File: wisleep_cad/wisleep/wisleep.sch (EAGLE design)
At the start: 23 parts, among them IC1 STM32F10XCXT6, U1 MAX1555, X1 8MHz

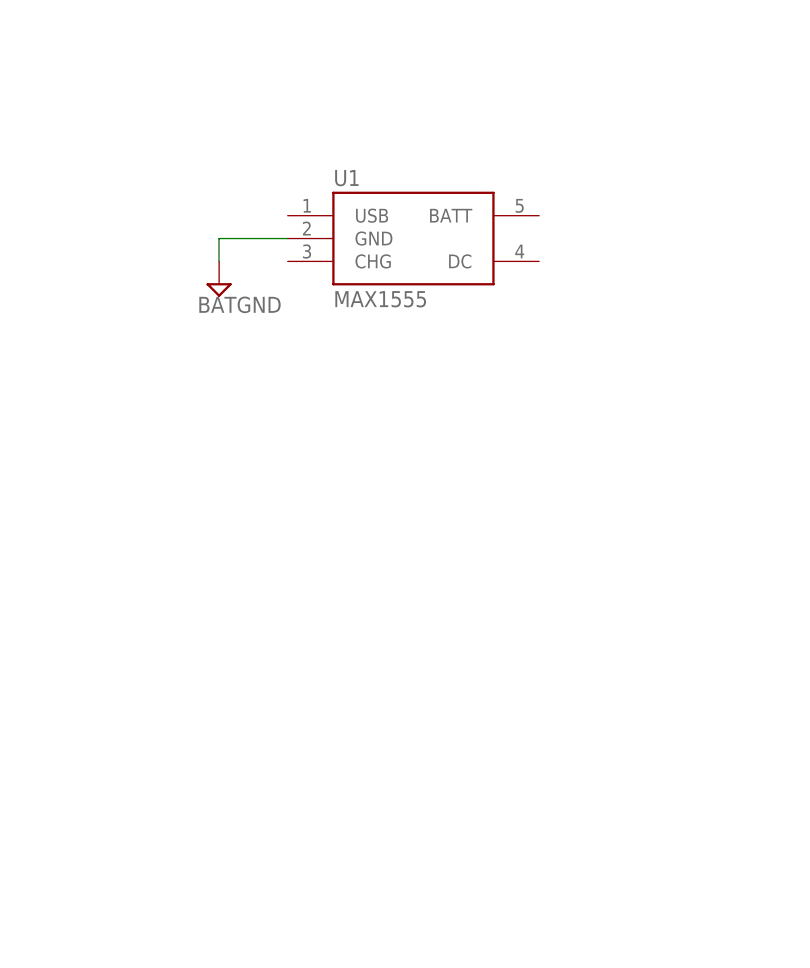
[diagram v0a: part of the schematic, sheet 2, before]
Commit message: some more cad
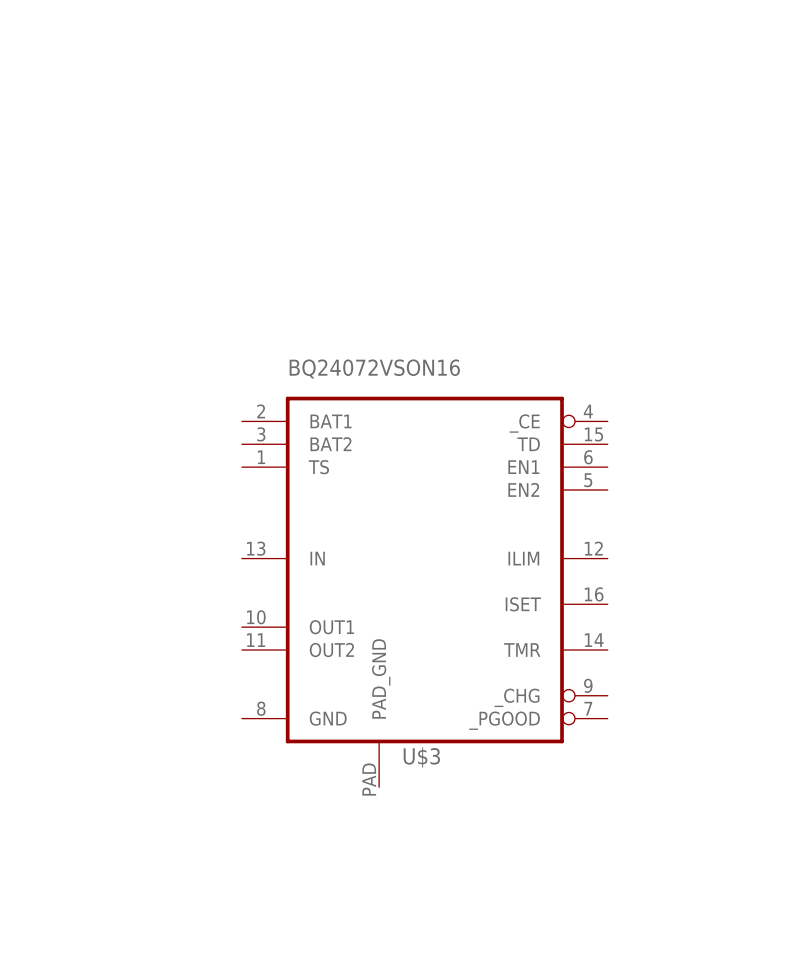
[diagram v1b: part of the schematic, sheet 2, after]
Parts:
- removed U1: MAX1555, SparkFun-PowerIC:MAX1555
- added U$3: BQ24072VSON16, robot:BQ24072VSON16
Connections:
- net GND2: no longer U1.GND
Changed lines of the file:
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@@
 <part name="SUPPLY2" library="SparkFun-Aesthetics" deviceset="3.3V" device=""/>
 <part name="GND7" library="SparkFun-Aesthetics" deviceset="GND" device=""/>
-<part name="U1" library="SparkFun-PowerIC" deviceset="MAX1555" device=""/>
 <part name="U$2" library="robot" deviceset="MAX8815A" device="MAX8815A" technology="OWN"/>
 <part name="MDL1" library="ESP8266-ESP12E" deviceset="ESP8266-12E" device="ESP8266-ESP12E"/>
@@
 <part name="GND6" library="SparkFun-Aesthetics" deviceset="GND" device=""/>
 <part name="SUPPLY4" library="supply2" deviceset="GND2" device="" value="BATGND"/>
-<part name="SUPPLY5" library="supply2" deviceset="GND2" device="" value="BATGND"/>
+<part name="U$3" library="robot" deviceset="BQ24072" device="VSON16"/>
 </parts>
 <sheets>
@@
 <instances>
 <instance part="GND7" gate="1" x="71.12" y="149.86"/>
-<instance part="U1" gate="G$1" x="71.12" y="116.84"/>
 <instance part="U$2" gate="G$1" x="71.12" y="170.18"/>
 <instance part="J1" gate="G$1" x="121.92" y="142.24"/>
@@
 <instance part="GND6" gate="1" x="129.54" y="132.08"/>
 <instance part="SUPPLY4" gate="G$1" x="137.16" y="132.08"/>
-<instance part="SUPPLY5" gate="G$1" x="48.26" y="111.76"/>
+<instance part="U$3" gate="G$1" x="71.12" y="78.74"/>
 </instances>
 <busses>
@@
 <junction x="132.08" y="142.24"/>
 </segment>
-<segment>
-<pinref part="U1" gate="G$1" pin="GND"/>
-<pinref part="SUPPLY5" gate="G$1" pin="GND2"/>
-<wire x1="55.88" y1="116.84" x2="48.26" y2="116.84" width="0.127" layer="91"/>
-<wire x1="48.26" y1="116.84" x2="48.26" y2="114.3" width="0.127" layer="91"/>
-</segment>
-</net>
+</net>

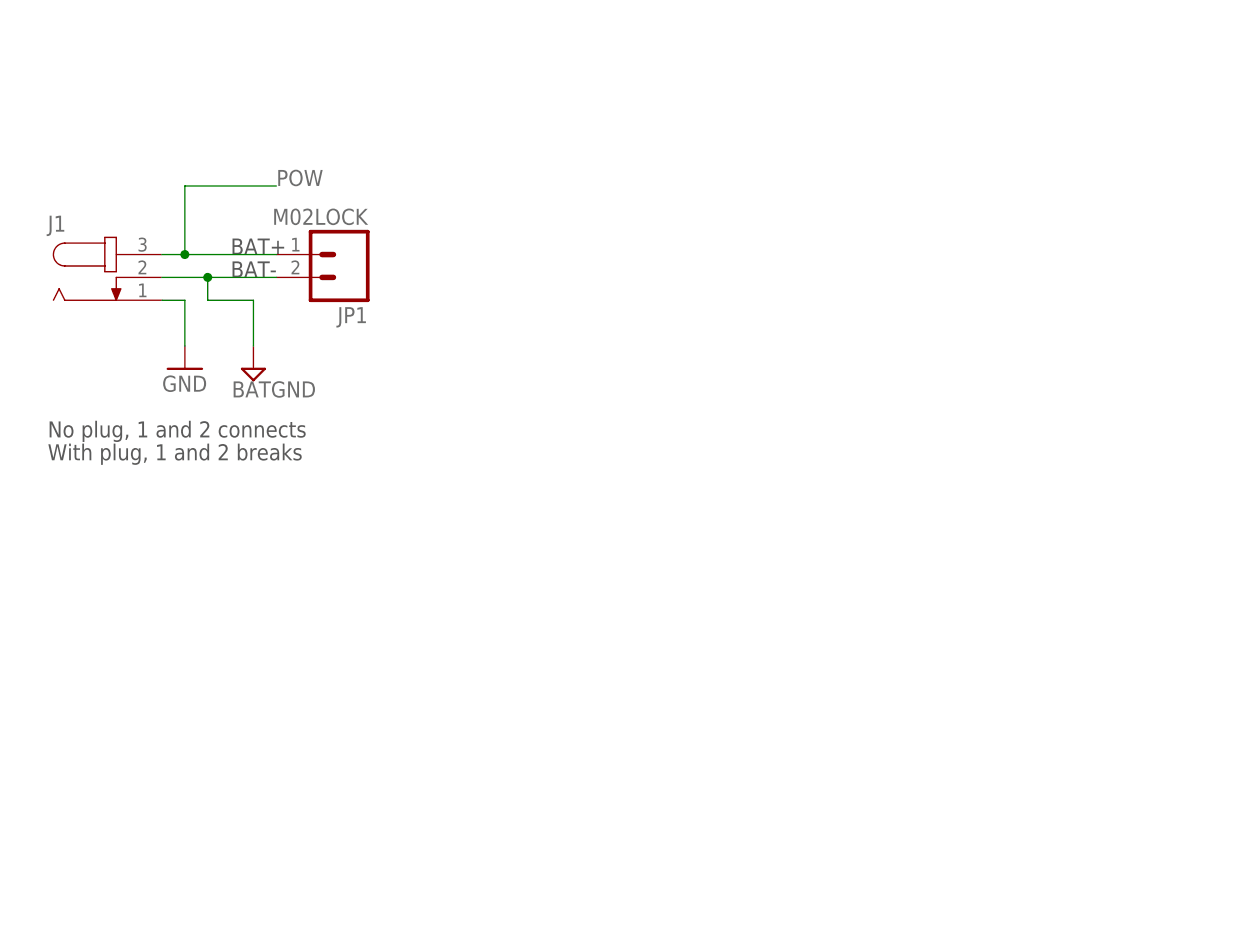
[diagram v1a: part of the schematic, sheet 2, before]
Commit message: more cadding
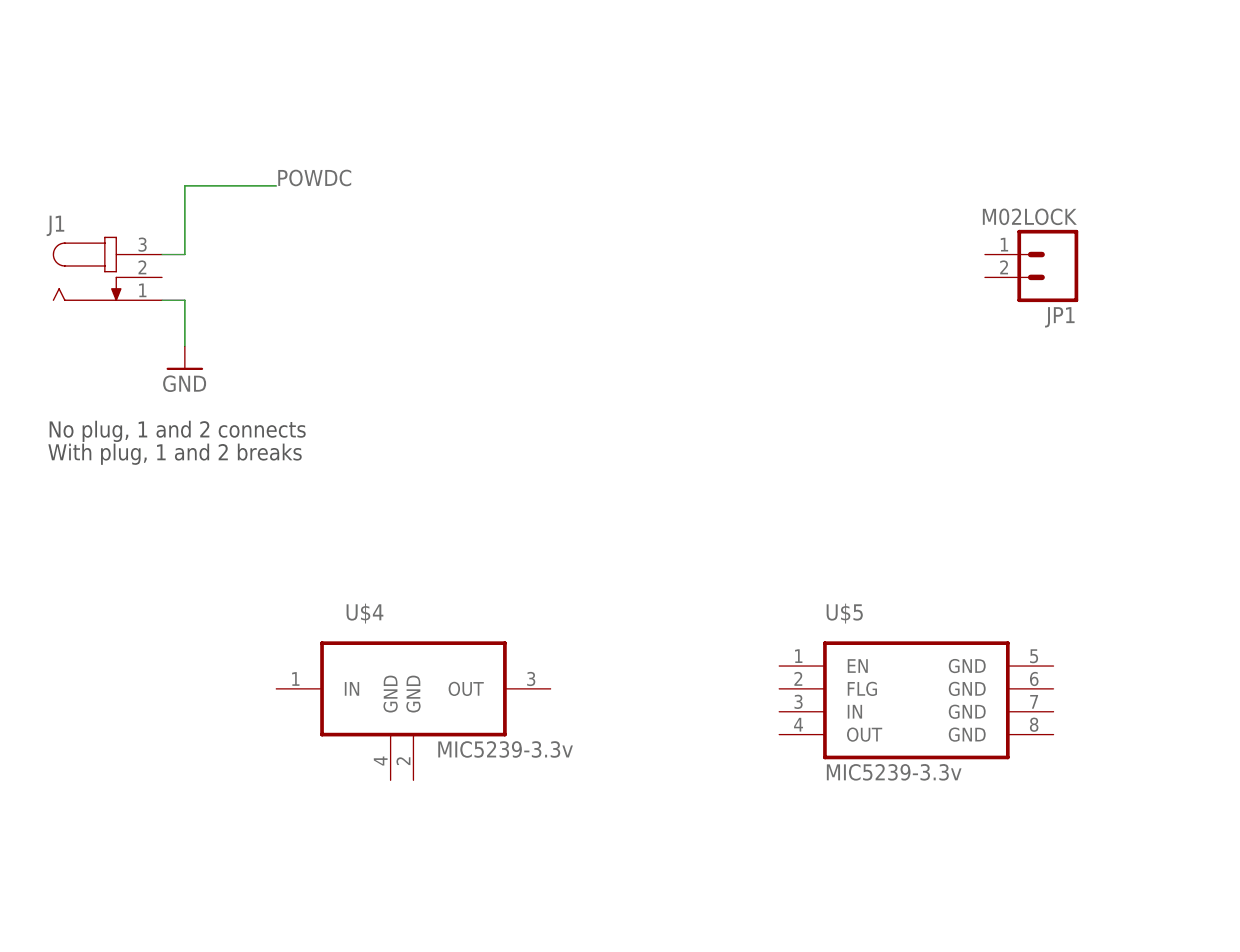
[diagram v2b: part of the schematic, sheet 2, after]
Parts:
- added U$4: MIC5239-3.3v, robot:MIC5239SOT223SOT223
- added U$5: MIC5239-3.3v, robot:MIC5239-8MSOP
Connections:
- net POW renamed POWDC
- removed net GND2: J1.2, JP1.2
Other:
- note removed: "BAT+"
- note removed: "BAT-"
- moved on the sheet: JP1
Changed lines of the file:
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@@
 <part name="JP1" library="SparkFun-Connectors" deviceset="M02" device="LOCK"/>
 <part name="GND6" library="SparkFun-Aesthetics" deviceset="GND" device=""/>
-<part name="SUPPLY4" library="supply2" deviceset="GND2" device="" value="BATGND"/>
 <part name="U$3" library="robot" deviceset="BQ24072" device="VSON16"/>
+<part name="U$4" library="robot" deviceset="MIC5239SOT223" device="SOT223" value="MIC5239-3.3v"/>
+<part name="U$5" library="robot" deviceset="MIC5239-8" device="MSOP" value="MIC5239-3.3v"/>
 </parts>
 <sheets>
@@
 <text x="195.58" y="17.78" size="1.778" layer="94">WISLEEP</text>
 <text x="195.58" y="10.16" size="1.778" layer="94">POWER</text>
-<text x="134.62" y="144.78" size="1.778" layer="97">BAT+</text>
-<text x="134.62" y="142.24" size="1.778" layer="97">BAT-</text>
 <text x="114.3" y="121.92" size="1.778" layer="97">With plug, 1 and 2 breaks</text>
 <text x="114.3" y="124.46" size="1.778" layer="97">No plug, 1 and 2 connects</text>
@@
 <instance part="U$2" gate="G$1" x="71.12" y="170.18"/>
 <instance part="J1" gate="G$1" x="121.92" y="142.24"/>
-<instance part="JP1" gate="G$1" x="147.32" y="144.78" rot="R180"/>
+<instance part="JP1" gate="G$1" x="226.06" y="144.78" rot="R180"/>
 <instance part="GND6" gate="1" x="129.54" y="132.08"/>
-<instance part="SUPPLY4" gate="G$1" x="137.16" y="132.08"/>
 <instance part="U$3" gate="G$1" x="71.12" y="78.74"/>
+<instance part="U$4" gate="G$1" x="154.94" y="96.52"/>
+<instance part="U$5" gate="G$1" x="210.82" y="93.98"/>
 </instances>
 <busses>
@@
 </segment>
 </net>
-<net name="POW" class="0">
+<net name="POWDC" class="0">
 <segment>
 <pinref part="J1" gate="G$1" pin="3"/>
 <wire x1="127" y1="144.78" x2="129.54" y2="144.78" width="0.127" layer="91"/>
-<wire x1="129.54" y1="144.78" x2="139.7" y2="144.78" width="0.127" layer="91"/>
 <wire x1="129.54" y1="144.78" x2="129.54" y2="152.4" width="0.127" layer="91"/>
-<junction x="129.54" y="144.78"/>
 <label x="139.7" y="152.4" size="1.778" layer="95"/>
 <wire x1="129.54" y1="152.4" x2="139.7" y2="152.4" width="0.127" layer="91"/>
 </segment>
 </net>
-<net name="GND2" class="0">
-<segment>
-<pinref part="J1" gate="G$1" pin="2"/>
-<pinref part="JP1" gate="G$1" pin="2"/>
-<wire x1="127" y1="142.24" x2="132.08" y2="142.24" width="0.127" layer="91"/>
-<wire x1="132.08" y1="142.24" x2="139.7" y2="142.24" width="0.127" layer="91"/>
-<wire x1="132.08" y1="142.24" x2="132.08" y2="139.7" width="0.127" layer="91"/>
-<wire x1="132.08" y1="139.7" x2="137.16" y2="139.7" width="0.127" layer="91"/>
-<wire x1="137.16" y1="139.7" x2="137.16" y2="134.62" width="0.127" layer="91"/>
-<pinref part="SUPPLY4" gate="G$1" pin="GND2"/>
-<junction x="132.08" y="142.24"/>
-</segment>
-</net>
